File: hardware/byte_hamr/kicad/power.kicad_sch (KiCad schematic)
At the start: 49 parts, among them U1 LFE5U-85F-8BG381I, U3 TLV62569DBV, U4 TLV62569DBV, U5 TLV62569DBV

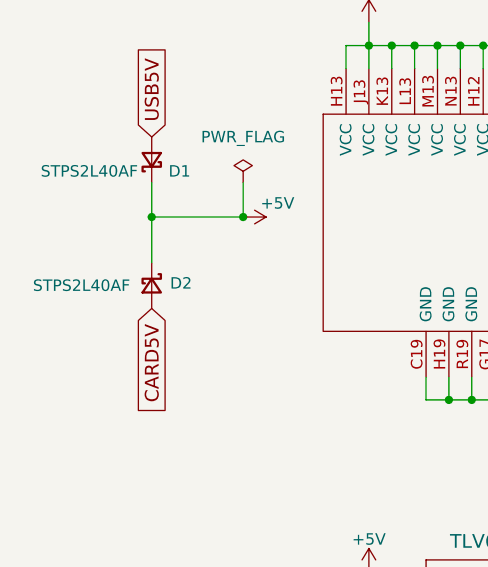
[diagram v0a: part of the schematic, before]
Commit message: Fabrication Feedback
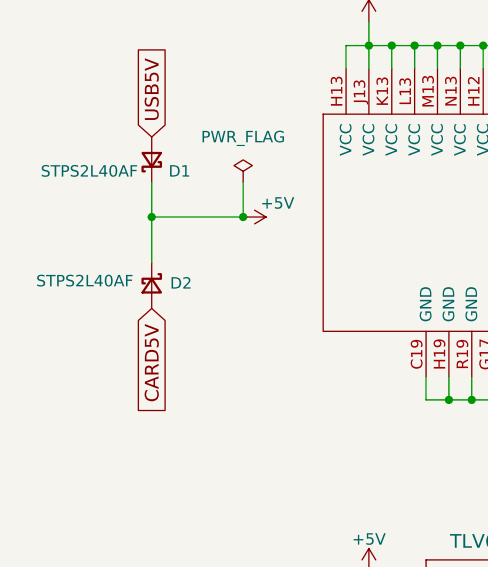
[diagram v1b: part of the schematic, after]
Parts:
- C1: Digike_y2 1276-2412-1-ND -> (none); Digikey 1276-2413-1-ND -> (none); Koncar FC004 -> (none); LCSC C29277 -> (none); MPN CC0805ZKY5V5BB226 -> CL21A226MQQNNNE; Mouse_r2 81-GRM21BR61A226ME1K -> (none); Mouse_r3 81-GRM219R61C226ME5L -> (none); Mouse_r4 81-GRM188C60J226ME0J -> (none); Mouse_r5 963-LMK212BBJ226MG-T -> (none); Mouser 81-GRM21BR61A226ME1L -> (none); Newark 08P5169 -> (none)
- C10, C6: MPN (none) -> FH 0603CG101J500NT
- C11, C12, C3, C4, C7, C8: MPN (none) -> CL21A226MQQNNNE
- C17, C19, C20, C22, C23, C24: MPN (none) -> CL21B225KOFNNNE
- C2: Digike_y2 399-9086-1-ND -> (none); Digikey 311-4078-1-ND -> (none); Koncar FC006 -> (none); LCSC C14665 -> (none); LCS_C2 C22396 -> (none); MNF1_URL www.yageo.com -> (none); MPN CS0603KRX7R9BB471 -> FH 0603CG101J500NT; Mouse_r1 710-885012206081 -> (none); Mouse_r2 603-CS0603KRX79BB471 -> (none); Mouse_r3 603-CC603JRNPO9BN101 -> (none); Mouse_r4 603-CC603KRX7R9BB471 -> (none); Mouser 581-06035A101JAT4A -> (none); Newark 38K9273 -> (none)
- C25: Digike_y2 1276-2000-1-ND -> (none); Digikey 587-1238-1-ND -> (none); Koncar FC003 -> (none); LCSC C107137 -> (none); MPN CC0603JRX7R8BB223 -> CX0603MRX7R8BB223; Mouse_r1 603-CC603JRX7R8BB223 -> (none); Mouse_r2 603-AC603KRX7R7BB223 -> (none); Mouse_r3 710-885012206091 -> (none); Mouser 603-CC603KRX7R7BB223 -> (none); Newark 82AC9346 -> (none); price1500_Mouser 35.7$ -> (none)
- C27, C28: MNF1_URL www.yageo.com -> (none)
- C5, C9: MPN CC0805ZKY5V5BB226 -> CL21A226MQQNNNE
- D1, D2: AvnetEU STPS2L30AF -> (none); Digikey 497-12310-1-ND -> (none); Koncar FV008 -> (none); LCSC C111630 -> (none); MNF1_URL www.st.com -> (none); MPN STPS2L30AF -> STPS2L40AF; Mouser 511-STPS2L40AF -> (none); Newark 69AH2828 -> (none); price100_AvnetEU 0.22121$ -> (none)
- L1: DatasheetLC https://datasheet.octopart.com/LQH32PB2R2NN0L-Murata-datash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 -> (none); Digike_y1 490-18405-1-ND -> (none); Digike_y2 490-10649-1-ND -> (none); Digikey 445-TFM322512ALMA2R2MTAACT-ND -> (none); Koncar FL001 -> (none); LCSC C285758 -> (none); LCS_C2 C285914 -> (none); LowCost 81-DFE252012P-2R2MP2 -> (none); MFG1 Murata -> (none); MFG2 Murata -> (none); MFG3 Bourns -> (none); MFG4 Chilisin Elec -> (none); MNF1_URL www.murata.com -> (none); MNF2_URL www.murata.com -> (none); MNF3_URL www.bourns.com -> (none); MPN DFE322512F-2R2M=P2 -> DFE322520FD-2R2M=P2; MP_N2 DFE252012P-2R2M=P2 -> (none); MP_N3 SRP2512A-2R2M -> (none); MP_N4 HEI322512A-2R2M-Q8 -> (none); MP_N5 81-LQH32PB2R2NN0L -> (none); Mouse_r1 710-74479299222 -> (none); Mouse_r2 810-TFM322512ALMA2R2 -> (none); Mouse_r3 81-DFE322520FD2R2MP2 -> (none); Mouser 81-DFE322512F-2R2MP2 -> (none); Newark 57AC6667 -> (none); Vertical DFE322512F-2R2M=P2 -> (none); price300_LCSC 0.1082$ -> (none); price300_Vertical 0.48360$ -> (none)
- L2, L3: MPN (none) -> DFE322520FD-2R2M=P2
- RA1: MNF1_URL www.yageo.com -> (none); MPN RC0603FR-1015KL -> RC0603FR-0715KL
- RA2, RA3: MPN (none) -> RC0603FR-0715KL
- RB1: Digikey 311-18.0KHRCT-ND -> (none); Koncar FR006 -> (none); LCSC C425614 -> (none); MNF1_URL www.yageo.com -> (none); Mouser 71-CRCW060318K0FKEAC -> (none); Newark 94X1474 -> (none)
- RB3: Digikey YAG3605CT-ND -> (none); Koncar FR009 -> (none); LCSC C425629 -> (none); MNF1_URL www.yageo.com -> (none); Mouse_r2 603-RC0603FR-103K3L -> (none); Mouser 603-RC0603FR-073K3L -> (none); Newark 94X1577 -> (none)
- RP1: Digike_y1 YAG1327CT-ND -> (none); EMPTY_MPN RC0805JR-070RL -> (none); MNF1_URL www.yageo.com -> (none); MPN (none) -> 0805W8F0000T5E; Mouse_r1 71-RCG08050000Z0EA -> (none); Mouse_r2 603-RC0805JR-070RL -> (none); Mouse_r3 652-CR0805-J/-000ELF -> (none); Mouser_URL www.mouser.com -> (none); Note Leave empty -> (none)
- RP2, RP3: MPN (none) -> 0805W8F0000T5E; Note Leave empty -> (none)
- U3: DatasheetLC http://www.dioo.com/attachments/files/20161031180022_361.pdf -> (none); Digikey 296-47360-1-ND -> (none); Koncar FU009 -> (none); LCSC C141836 -> (none); LowCost 453-DIO6015BCST5 -> (none); MFG1 TI -> (none); MFG2 DIOO -> (none); MNF1_URL www.ti.com -> (none); MNF2_URL www.dioo.com -> (none); MPN2 DIO6015BCST5 -> (none); Mouse_r0 595-TLV62569DBVT -> (none); Mouse_r1 595-TLV62569DBVR -> (none); Mouse_r2 595-TLV62566DBVR -> (none); Mouse_r3 595-TLV62565DBVR -> (none); Mouse_r4 453-DIO6012BCST6 -> (none); Mouse_r5 453-DIO6015BCST5 -> (none); Mouser 453-DIO6015BCST5 -> (none); Newark 54AH1585 -> (none); price100_LCSC 0.1843$ -> (none)
- U4, U5: MNF1_URL www.ti.com -> (none); Mouser 595-TLV62569DBVR -> (none)
